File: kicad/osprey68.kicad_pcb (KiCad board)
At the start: 2 copper layers, 150 x 92 mm, 65 parts, among them J1 PS2_USB, J2 Conn_01x08_Pin, J3 AVR-ISP-6, J4 Conn_01x04_Pin, J6 SD, J7 I2c, J8 LCD, Q1 AO3401A, Q10 AO3400A, Q11 AO3401A, Q12 AO3400A, Q13 AO3401A, Q14 AO3400A, Q15 AO3401A, Q16 AO3400A, Q2 AO3400A, Q3 AO3401A, Q4 AO3400A, Q5 AO3401A, Q6 AO3400A, Q7 AO3401A, Q8 AO3400A, Q9 AO3401A, SW1 SW_Push, SW2 SW_SPDT, U1 MC6809E, U10 ATmega16A-P, U11 W65C22NxP, U12 AMS1117-3.3, U15 W65C22NxP, U2 74HC74, U3 28C256, U4 74HC245D, U5 GAL20V8, U6 74HC245D, U7 74HC245D, U8 HM628128D_DIP32_SOP32, U9 CY62256-70PC, Y1 8Mhz, Y2 16Mhz

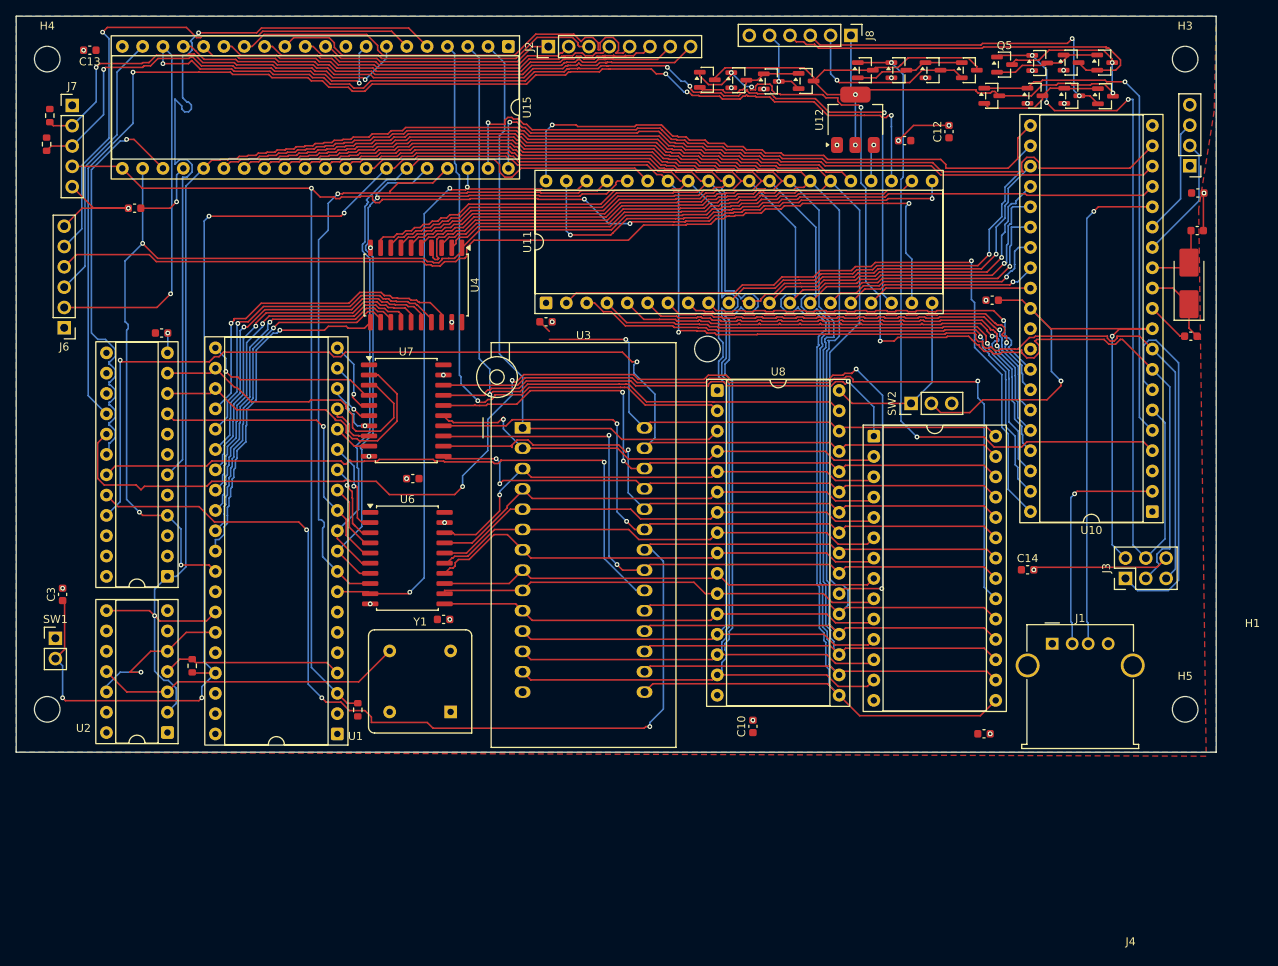
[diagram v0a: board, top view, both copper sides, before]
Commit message: add third menu
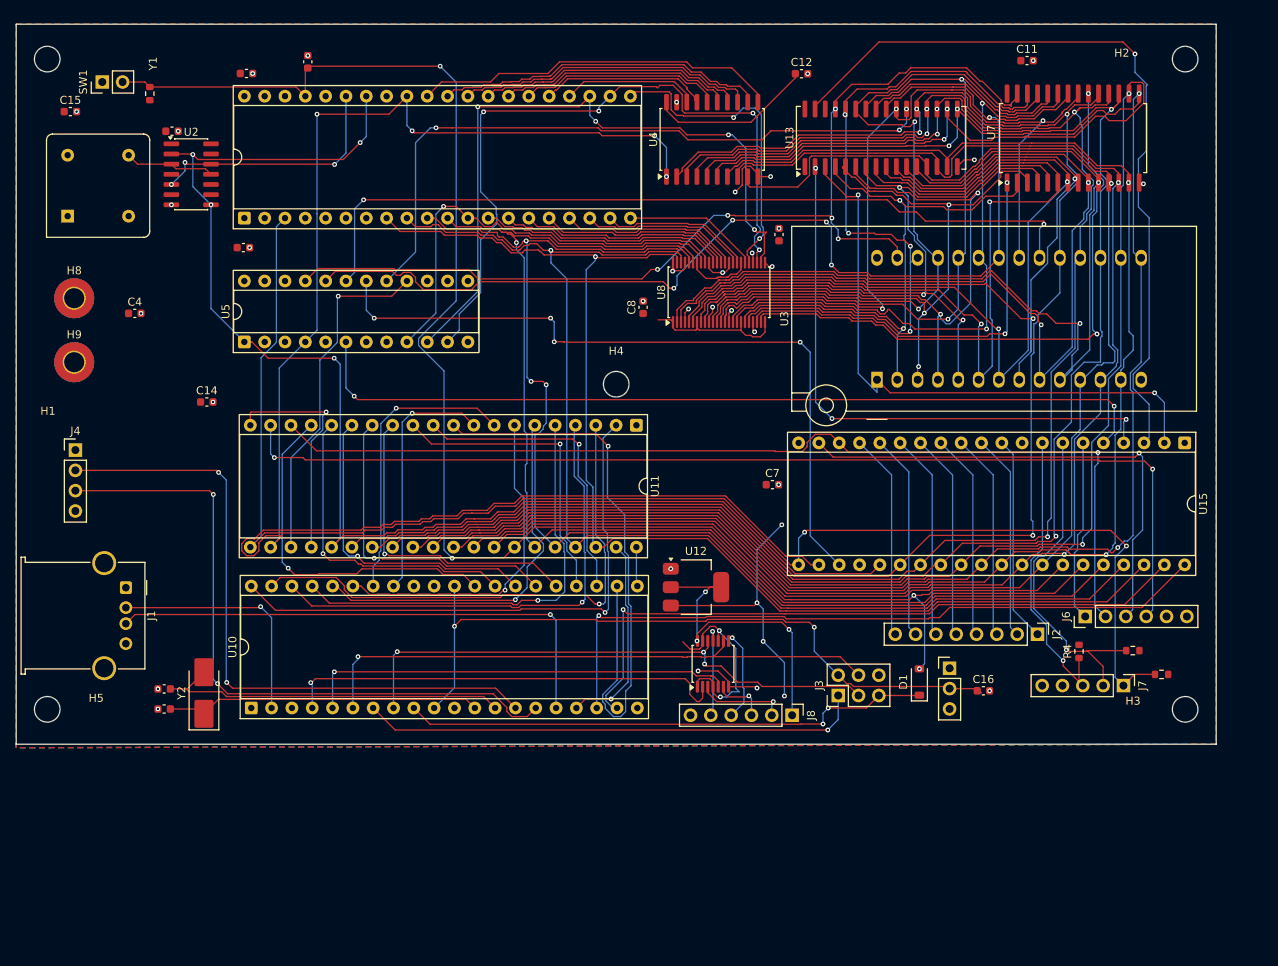
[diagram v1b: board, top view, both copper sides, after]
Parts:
- removed C10: 100n, Capacitor_SMD:C_0603_1608Metric
- removed Q1, Q11, Q13, Q15, Q3, Q5, Q7, Q9: AO3401A, Package_TO_SOT_SMD:SOT-23
- removed Q10, Q12, Q14, Q16, Q2, Q4, Q6, Q8: AO3400A, Package_TO_SOT_SMD:SOT-23
- removed U9: CY62256-70PC, Package_DIP:DIP-28_W15.24mm_Socket
- added D1: 1N4148W, Diode_SMD:D_SOD-123, F.Cu at (157.2, 117.1)
- added H8: +5v, MountingHole:MountingHole_2.5mm_Pad_TopBottom, F.Cu at (51.6, 69.2)
- added H9: GND, MountingHole:MountingHole_2.5mm_Pad_TopBottom, F.Cu at (51.6, 77.2)
- added U13: ~, Package_SO:SOJ-32_7.62x20.955mm_P1.27mm, F.Cu at (152.5, 49.1)
- U11: value W65C22NxP -> VIA0
- U15: value W65C22NxP -> VIA1
- U2: footprint Package_DIP:DIP-14_W7.62mm_Socket -> Package_SO:SO-14_3.9x8.65mm_P1.27mm
- U6: value 74HC245D -> SN74LVC126APWR-TP; footprint Package_SO:SOIC-20W_7.5x12.8mm_P1.27mm -> Package_SO:TSSOP-14_4.4x5mm_P0.65mm
- U7: value 74HC245D -> IS62C256AL; footprint Package_SO:SOIC-20W_7.5x12.8mm_P1.27mm -> Package_SO:SOP-28_8.4x18.16mm_P1.27mm
- U8: value HM628128D_DIP32_SOP32 -> SN74AHCT16245DGGR; footprint Package_DIP:DIP-32_W15.24mm_Socket -> Package_SO:TSSOP-48_6.1x12.5mm_P0.5mm
- moved R3 151.0 mm to (183.9, 113.2), turned to 0 degrees
- moved J7 150.1 mm to (182.7, 117.6), turned to -90 degrees
- moved R4 143.8 mm to (177.2, 113.3)
- moved J4 143.8 mm to (51.7, 88.1), turned to 0 degrees
- moved H5 142.2 mm to (48.2, 120.6)
- moved C1 141.3 mm to (62.8, 118.0), turned to 0 degrees
- moved C2 136.5 mm to (62.8, 120.5)
- moved Y2 133.4 mm to (67.8, 118.5)
- moved J6 132.6 mm to (178.0, 108.9), turned to 90 degrees
- moved C6 126.4 mm to (63.8, 48.3)
- moved J1 116.0 mm to (58.0, 105.3), turned to -90 degrees
- moved U10 115.3 mm to (73.7, 120.4), turned to 90 degrees
- moved C11 113.1 mm to (170.7, 39.5), turned to 0 degrees
- moved C14 104.7 mm to (68.2, 82.1)
- moved R2 100.6 mm to (187.5, 116.2), turned to 0 degrees
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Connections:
- net Net-(J7-Pin_2) renamed /peripheral/SCL
- net Net-(J7-Pin_3) renamed /peripheral/SDA
- J3 pad 5: ~{RESET} -> ~{AVRRESET}
- J6 pad 1: +5V -> /peripheral/SD_CS
- J6 pad 5: /peripheral/SD_CS -> +5V
- J7 pad 1: +5V -> ~{IRQ}
- J7 pad 4: ~{IRQ} -> +5V
- U10 pad 4: /peripheral/logicshift3/in -> Net-(U10-PB3)
- U10 pad 5: /peripheral/logicshift2/in -> Net-(U10-PB4)
- U10 pad 9: ~{RESET} -> ~{AVRRESET}
- U6 pad 10: GND -> +5V
- U6 pad 11: /memory/A0 -> /peripheral/LCD_CK
- U6 pad 12: /memory/A1 -> /peripheral/SCK
- U6 pad 13: /memory/A2 -> +5V
- U6 pad 14: /memory/A3 -> +3.3V
- U6 pad 2: CPU_A7 -> Net-(U10-PB3)
- U6 pad 3: CPU_A6 -> /peripheral/LCD_DC
- U6 pad 4: CPU_A5 -> +5V
- U6 pad 5: CPU_A4 -> Net-(U10-PB4)
- U6 pad 6: CPU_A3 -> /peripheral/LCD_CS
- U6 pad 7: CPU_A2 -> GND
- U6 pad 8: CPU_A1 -> /peripheral/LCD_MOSI
- U6 pad 9: CPU_A0 -> /peripheral/MOSI
- U7 pad 1: +5V -> /memory/A14
- U7 pad 10: GND -> /memory/A0
- U7 pad 11: /memory/A8 -> P_0
- U7 pad 12: /memory/A9 -> P_1
- U7 pad 13: /memory/A10 -> P_2
- U7 pad 14: /memory/A11 -> GND
- U7 pad 15: /memory/A12 -> P_3
- U7 pad 16: /memory/A13 -> P_4
- U7 pad 17: /memory/A14 -> P_5
- U7 pad 18: /memory/A15 -> P_6
- U7 pad 19: GND -> P_7
- U7 pad 2: CPU_A15 -> /memory/A12
- U7 pad 20: +5V -> /memory/A15
- U7 pad 3: CPU_A14 -> /memory/A7
- U7 pad 4: CPU_A13 -> /memory/A6
- U7 pad 5: CPU_A12 -> /memory/A5
- U7 pad 6: CPU_A11 -> /memory/A4
- U7 pad 7: CPU_A10 -> /memory/A3
- U7 pad 8: CPU_A9 -> /memory/A2
- U7 pad 9: CPU_A8 -> /memory/A1
- U8 pad 1: unconnected-(U8-NC-Pad1) -> +5V
- U8 pad 10: /memory/A2 -> GND
- U8 pad 11: /memory/A1 -> /memory/A6
- U8 pad 12: /memory/A0 -> /memory/A7
- U8 pad 13: P_0 -> /memory/A8
- U8 pad 14: P_1 -> /memory/A9
- U8 pad 15: P_2 -> GND
- U8 pad 16: GND -> /memory/A10
- U8 pad 17: P_3 -> /memory/A11
- U8 pad 18: P_4 -> +5V
- U8 pad 19: P_5 -> /memory/A12
- U8 pad 2: SEL2 -> /memory/A0
- U8 pad 20: P_6 -> /memory/A13
- U8 pad 21: P_7 -> GND
- U8 pad 22: ~{HIRAMCS} -> /memory/A14
- U8 pad 23: /memory/A10 -> /memory/A15
- U8 pad 24: ~{RD} -> +5V
- U8 pad 25: /memory/A11 -> GND
- U8 pad 26: /memory/A9 -> CPU_A15
- U8 pad 27: /memory/A8 -> CPU_A14
- U8 pad 28: /memory/A13 -> GND
- U8 pad 29: ~{WR} -> CPU_A13
- U8 pad 3: SEL0 -> /memory/A1
- U8 pad 30: +5V -> CPU_A12
- U8 pad 31: SEL1 -> +5V
- U8 pad 32: +5V -> CPU_A11
- U8 pad 4: /memory/A12 -> GND
- U8 pad 5: /memory/A7 -> /memory/A2
- U8 pad 6: /memory/A6 -> /memory/A3
- U8 pad 7: /memory/A5 -> +5V
- U8 pad 9: /memory/A3 -> /memory/A5
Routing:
- net ~{IO2CS}: track 154.0 -> 43.2 mm, vias 4 -> 1
- net /peripheral/logicshift3/in: track 83.2 -> 0.00 mm, vias 2 -> 0
- net +3.3V: track 109.3 -> 39.3 mm, vias 4 -> 3
- net CPU_A0: track 81.9 -> 151.7 mm, vias 3 -> 1
- net /peripheral/SR_TX: track 14.7 -> 83.5 mm, vias 0 -> 2
- net /peripheral/AC2: track 73.5 -> 4.75 mm, vias 1 -> 0
- net ~{RESET}: track 270.9 -> 203.3 mm, vias 5 -> 4
- net /peripheral/SR_RX: track 15.6 -> 82.1 mm, vias 0 -> 2
- net ~{AVRRESET}: track 0.00 -> 66.3 mm, vias 0 -> 2
- net ~{HIRAMCS}: track 148.8 -> 84.2 mm, vias 4 -> 3
- net /memory/A0: track 54.8 -> 118.8 mm, vias 0 -> 2
- net /peripheral/logicshift2/in: track 63.1 -> 0.00 mm, vias 1 -> 0
- net CPU_A2: track 92.9 -> 154.1 mm, vias 1 -> 3
- net CPU_A3: track 90.3 -> 150.6 mm, vias 0 -> 1
- net /memory/A1: track 55.1 -> 113.0 mm, vias 0 -> 2
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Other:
- board size 150 x 92 mm -> 150 x 90 mm
